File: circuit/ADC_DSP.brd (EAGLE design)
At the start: 43.5 x 55.2 mm, 49 parts, among them IC1 REG1117, IC2 AD8605, IC3 STM32F40XRXT6, IC4 CS4272, Q1 8MHz, Q2 24.576MHz

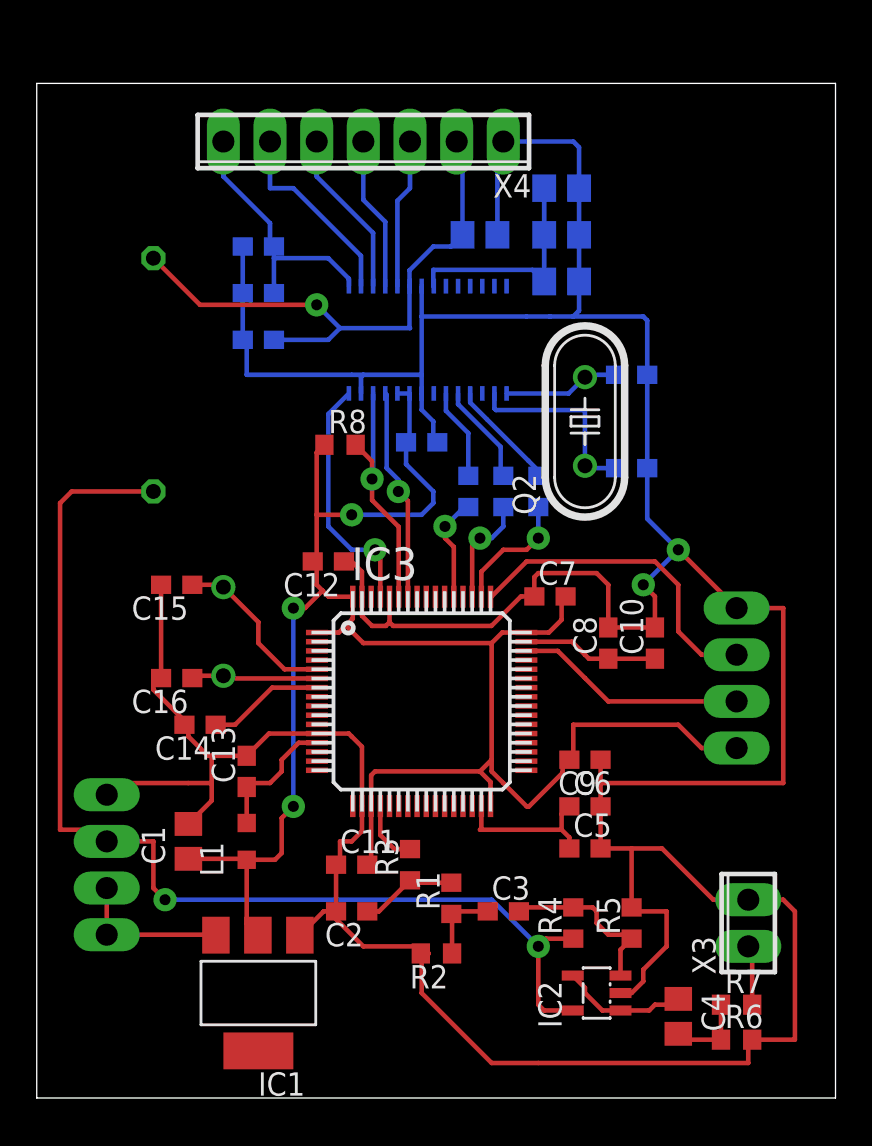
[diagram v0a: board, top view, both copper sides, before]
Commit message: - ???????? ???????????? (??????? ????? ? ?? ????? ???????)
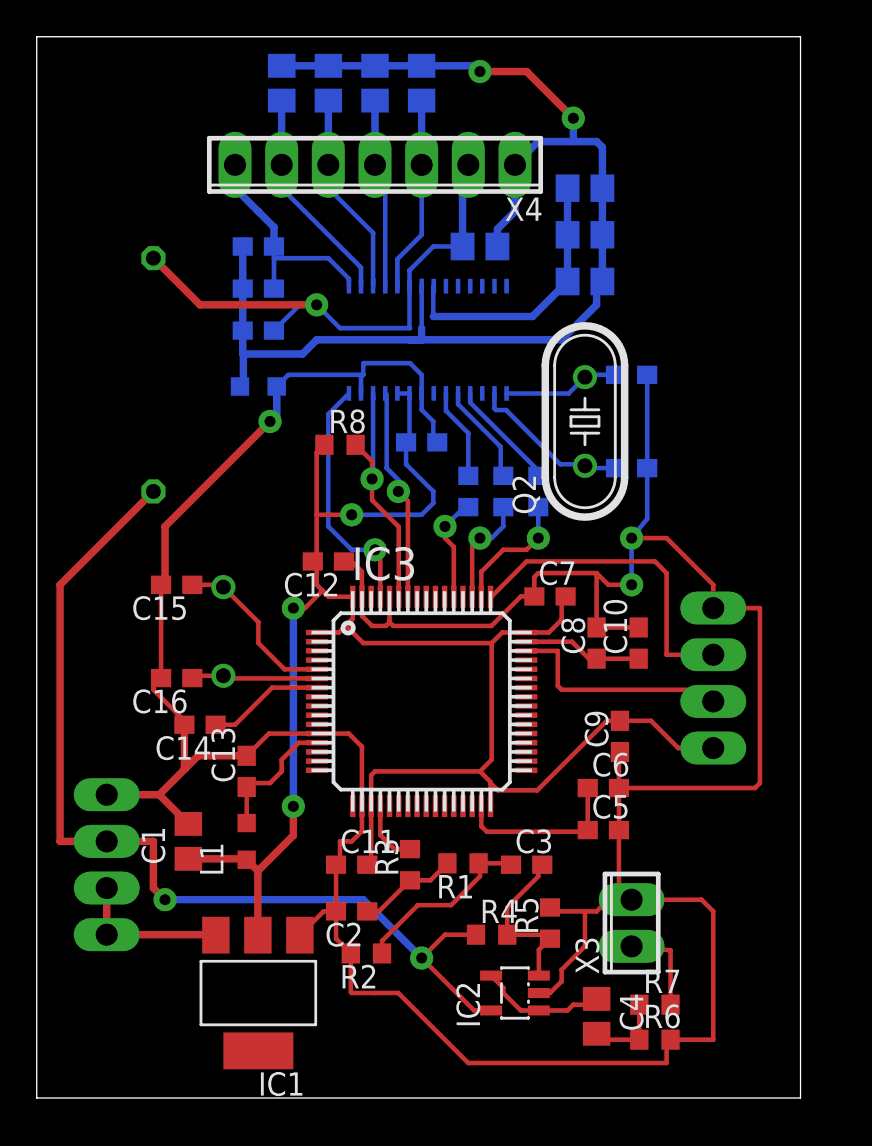
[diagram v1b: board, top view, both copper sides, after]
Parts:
- added C27, C28, C29, C30: (no value), rcl:C0805
- added L3: (no value), rcl:L2012C
- moved X3 6.35 mm to (32.4, 9.53)
- moved R4 4.49 mm to (24.8, 8.89), turned to 0 degrees
- moved IC2 4.45 mm to (26.0, 5.71)
- moved R6 4.45 mm to (33.7, 3.17)
- moved R7 4.45 mm to (33.7, 5.08)
- moved C4 4.44 mm to (30.5, 4.45)
- moved R5 4.44 mm to (27.9, 9.53)
- moved R2 3.81 mm to (17.9, 7.87)
- moved C3 2.84 mm to (26.7, 12.7)
- moved C9 2.29 mm to (31.8, 19.7), turned to 90 degrees
- moved R1 2.01 mm to (23.2, 12.8), turned to 180 degrees
- moved X4 1.42 mm to (18.4, 50.8)
- moved C5 1.41 mm to (30.8, 14.6)
- moved C6 1.41 mm to (30.8, 16.9)
- moved X2 1.27 mm to (36.8, 22.9)
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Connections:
- net N$13 renamed VCOM
- net N$14 renamed AVCC
- new net AGND: C20.2, C21.2, C22.2, C23.2, C24.2, C25.2, C26.2, C27.2, C28.2, C29.2, C30.2, IC4.21, L3.2, X4.1
- net GND: now also L3.1; no longer C20.2, C21.2, C22.2, C23.2, C24.2, C25.2, C26.2, IC4.21, X4.1
- net N$15: now also C30.1
- net N$16: now also C29.1
- net N$17: now also C28.1
- net N$18: now also C27.1
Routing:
- net AGND: track 0.00 -> 69.3 mm, vias 0 -> 2
- net GND: track 238.0 -> 191.9 mm, vias 2 -> 3
- net +5V: track 60.5 -> 53.4 mm
- net N$24: track 4.20 -> 10.0 mm
- net +3V3: track 105.8 -> 101.4 mm
- net N$12: track 12.3 -> 14.8 mm
- net N$15: track 8.16 -> 10.6 mm
- net N$16: track 8.37 -> 10.3 mm
- net N$17: track 9.15 -> 11.1 mm
- net AVCC: track 31.5 -> 29.6 mm
- net N$21: track 3.26 -> 5.09 mm
- net N$7: track 10.6 -> 8.78 mm
- net VCOM: track 14.3 -> 12.6 mm
- net N$18: track 10.7 -> 11.9 mm
- net N$2: track 8.40 -> 9.33 mm
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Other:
- board size 43.5 x 55.2 mm -> 41.6 x 57.8 mm
